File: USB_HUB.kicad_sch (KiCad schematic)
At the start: 2 parts, among them U1 TUSB8043A, Y1 Crystal_GND24

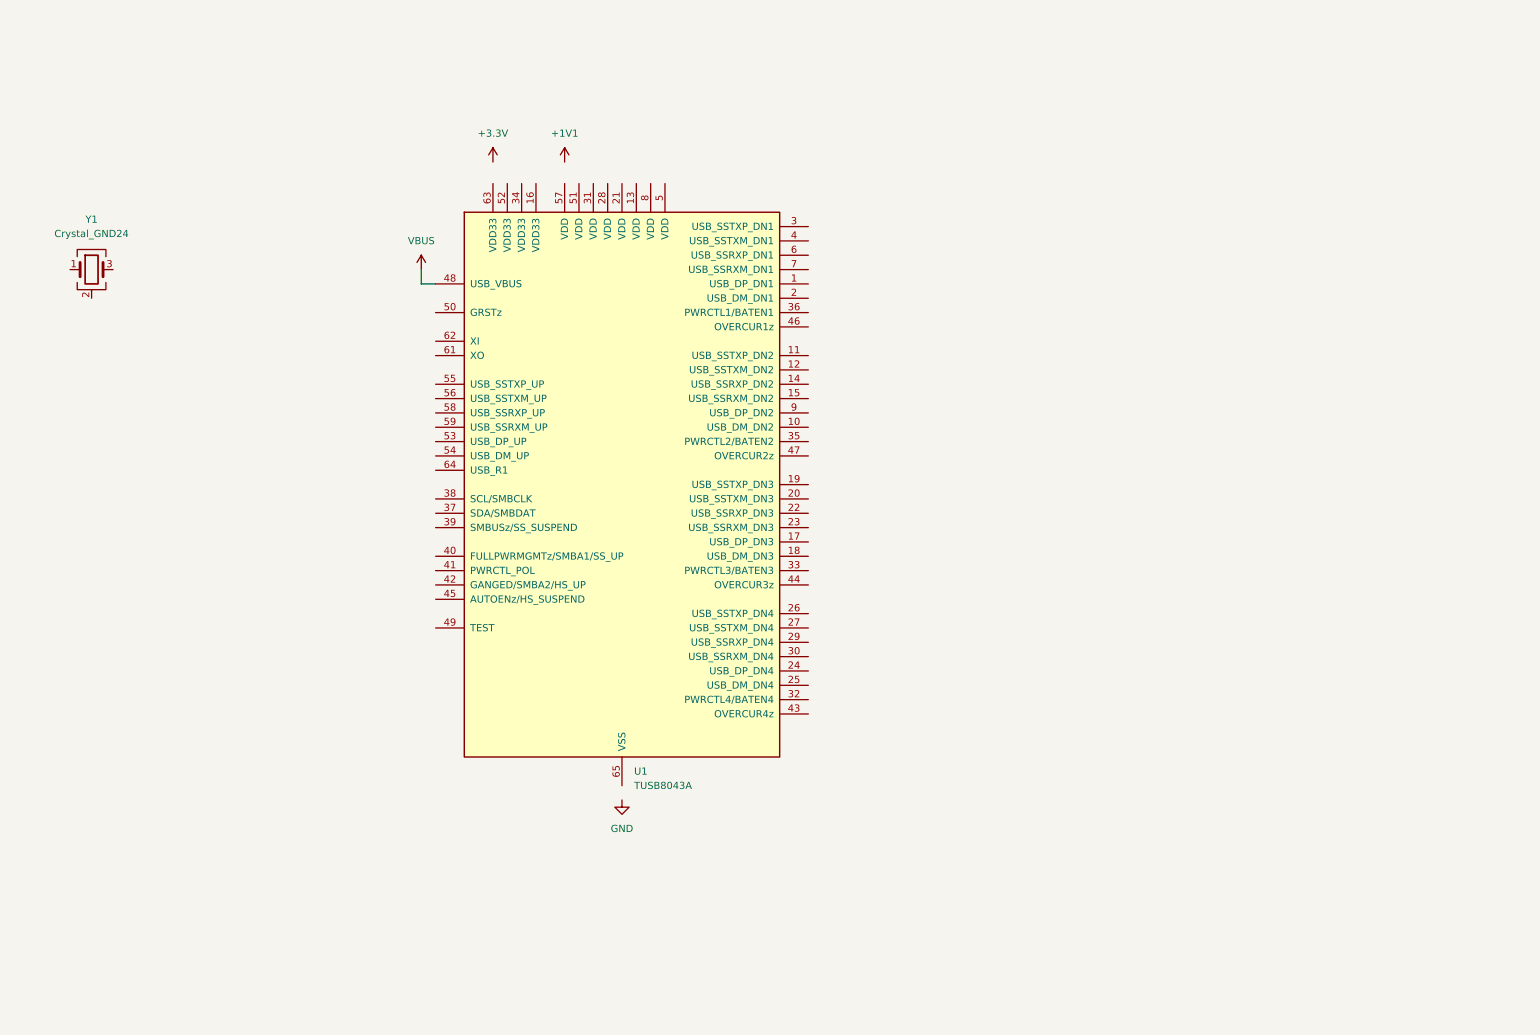
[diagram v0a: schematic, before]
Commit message: Weiter gearbeitet
Fast fertig:
HUB
Fertig
Connector (Up and Down)
MUX
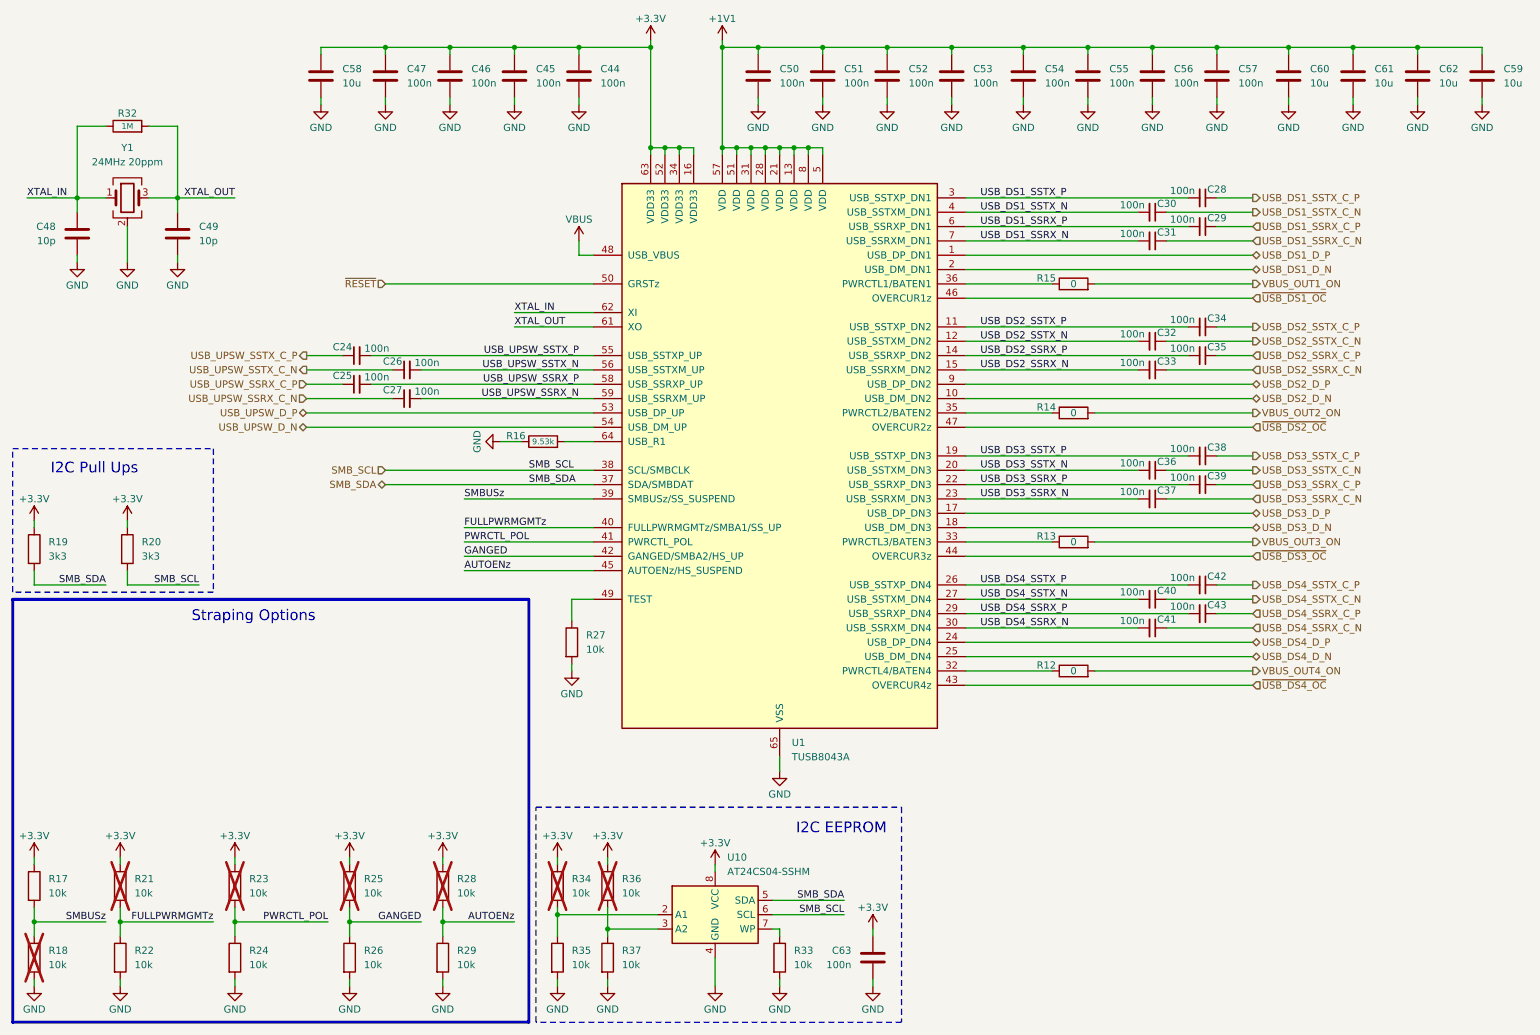
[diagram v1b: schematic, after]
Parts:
- added C24, C25, C26, C27, C28, C29, C30, C31, C32, C33, C34, C35, C36, C37, C38, C39, C40, C41, C42, C43: 100n, symbol Device:C_Small
- added C44, C45, C46, C47, C50, C51, C52, C53, C54, C55, C56, C57, C63: 100n, Capacitor_SMD:C_0402_1005Metric, symbol Device:C
- added C48, C49: 10p, Capacitor_SMD:C_0402_1005Metric, symbol Device:C
- added C58, C59, C60, C61, C62: 10u, Capacitor_SMD:C_0603_1608Metric, symbol Device:C
- added R12, R13, R14, R15: 0, Resistor_SMD:R_0402_1005Metric, symbol Device:R
- added R16: 9.53k, Resistor_SMD:R_0402_1005Metric, symbol Device:R
- added R17, R18, R21, R22, R23, R24, R25, R26, R27, R28, R29, R33, R34, R35, R36, R37: 10k, Resistor_SMD:R_0402_1005Metric, symbol Device:R
- added R19, R20: 3k3, Resistor_SMD:R_0402_1005Metric, symbol Device:R
- added R32: 1M, Resistor_SMD:R_0402_1005Metric, symbol Device:R
- added U10: AT24CS04-SSHM, Package_SO:SOIC-8_3.9x4.9mm_P1.27mm, symbol Memory_EEPROM:AT24CS04-SSHM
- Y1: value Crystal_GND24 -> 24MHz 20ppm
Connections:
- net +1V1: now also U1.13 (VDD), U1.21 (VDD), U1.28 (VDD), U1.31 (VDD), U1.5 (VDD), U1.51 (VDD), U1.57 (VDD), U1.8 (VDD), C50.2, C51.2, C52.2, C53.2, C54.2, C55.2, C56.2, C57.2, C59.1, C60.1, C61.1, C62.1
- net +3.3V: now also U1.16 (VDD33), U1.34 (VDD33), U1.52 (VDD33), U1.63 (VDD33), C44.2, C45.2, C46.2, C47.2, C58.1, C63.2, R17.1, R19.1, R20.1, R21.1, R23.1, R25.1, R28.1, R34.1, R36.1, U10.8 (VCC)
- net GND: now also U1.65 (VSS), Y1.2 (G), Y1.4 (G), C44.1, C45.1, C46.1, C47.1, C48.1, C49.1, C50.1, C51.1, C52.1, C53.1, C54.1, C55.1, C56.1, C57.1, C58.2, C59.2, C60.2, C61.2, C62.2, C63.1, R16.1, R18.2, R22.2, R24.2, R26.2, R27.2, R29.2, R33.2, R35.2, R37.2, U10.4 (GND)
- net USB_DS1_D_P: now reaches U1.1 (USB_DP_DN1)
- net USB_DS2_D_N: now reaches U1.10 (USB_DM_DN2)
- net USB_DS2_SSTX_P: now reaches U1.11 (USB_SSTXP_DN2)
- net USB_DS2_SSTX_P: now also C34.2
- net USB_DS2_SSTX_N: now reaches U1.12 (USB_SSTXM_DN2)
- net USB_DS2_SSTX_N: now also C32.2
- net USB_DS2_SSRX_P: now reaches U1.14 (USB_SSRXP_DN2)
- net USB_DS2_SSRX_P: now also C35.2
- net USB_DS2_SSRX_N: now reaches U1.15 (USB_SSRXM_DN2)
- net USB_DS2_SSRX_N: now also C33.2
- net USB_DS3_D_P: now reaches U1.17 (USB_DP_DN3)
- net USB_DS3_D_N: now reaches U1.18 (USB_DM_DN3)
- net USB_DS3_SSTX_P: now reaches U1.19 (USB_SSTXP_DN3)
- net USB_DS3_SSTX_P: now also C38.2
- net USB_DS1_D_N: now reaches U1.2 (USB_DM_DN1)
- net USB_DS3_SSTX_N: now reaches U1.20 (USB_SSTXM_DN3)
- net USB_DS3_SSTX_N: now also C36.2
- net USB_DS3_SSRX_P: now reaches U1.22 (USB_SSRXP_DN3)
- net USB_DS3_SSRX_P: now also C39.2
- net USB_DS3_SSRX_N: now reaches U1.23 (USB_SSRXM_DN3)
- net USB_DS3_SSRX_N: now also C37.2
- net USB_DS4_D_P: now reaches U1.24 (USB_DP_DN4)
- net USB_DS4_D_N: now reaches U1.25 (USB_DM_DN4)
- net USB_DS4_SSTX_P: now reaches U1.26 (USB_SSTXP_DN4)
- net USB_DS4_SSTX_P: now also C42.2
- net USB_DS4_SSTX_N: now reaches U1.27 (USB_SSTXM_DN4)
- net USB_DS4_SSTX_N: now also C40.2
- net USB_DS4_SSRX_P: now reaches U1.29 (USB_SSRXP_DN4)
- net USB_DS4_SSRX_P: now also C43.2
- net USB_DS1_SSTX_P: now reaches U1.3 (USB_SSTXP_DN1)
- net USB_DS1_SSTX_P: now also C28.2
- net USB_DS4_SSRX_N: now reaches U1.30 (USB_SSRXM_DN4)
- net USB_DS4_SSRX_N: now also C41.2
- net at U1.32 (PWRCTL4/BATEN4): now also R12.1
- net at U1.33 (PWRCTL3/BATEN3): now also R13.1
- net at U1.35 (PWRCTL2/BATEN2): now also R14.1
- net at U1.36 (PWRCTL1/BATEN1): now also R15.1
- net SMB_SDA: now reaches U1.37 (SDA/SMBDAT)
- net SMB_SDA: now also R19.2, U10.5 (SDA)
- net SMB_SCL: now reaches U1.38 (SCL/SMBCLK)
- net SMB_SCL: now also R20.2, U10.6 (SCL)
- net SMBUSz: now reaches U1.39 (SMBUSz/SS_SUSPEND)
- net SMBUSz: now also R17.2, R18.1
- net USB_DS1_SSTX_N: now reaches U1.4 (USB_SSTXM_DN1)
- net USB_DS1_SSTX_N: now also C30.2
- net FULLPWRMGMTz: now reaches U1.40 (FULLPWRMGMTz/SMBA1/SS_UP)
- net FULLPWRMGMTz: now also R21.2, R22.1
- net PWRCTL_POL: now reaches U1.41 (PWRCTL_POL)
- net PWRCTL_POL: now also R23.2, R24.1
- net GANGED: now reaches U1.42 (GANGED/SMBA2/HS_UP)
- net GANGED: now also R25.2, R26.1
- net ~{USB_DS4_OC}: now reaches U1.43 (OVERCUR4z)
- net ~{USB_DS3_OC}: now reaches U1.44 (OVERCUR3z)
- net AUTOENz: now reaches U1.45 (AUTOENz/HS_SUSPEND)
- net AUTOENz: now also R28.2, R29.1
- net ~{USB_DS1_OC}: now reaches U1.46 (OVERCUR1z)
- net ~{USB_DS2_OC}: now reaches U1.47 (OVERCUR2z)
- net at U1.49 (TEST): now also R27.1
- net ~{RESET}: now reaches U1.50 (GRSTz)
- net USB_UPSW_D_P: now reaches U1.53 (USB_DP_UP)
- net USB_UPSW_D_N: now reaches U1.54 (USB_DM_UP)
- net USB_UPSW_SSTX_P: now reaches U1.55 (USB_SSTXP_UP)
- net USB_UPSW_SSTX_P: now also C24.2
- net USB_UPSW_SSTX_N: now reaches U1.56 (USB_SSTXM_UP)
- net USB_UPSW_SSTX_N: now also C26.2
- net USB_UPSW_SSRX_P: now reaches U1.58 (USB_SSRXP_UP)
- net USB_UPSW_SSRX_P: now also C25.2
- net USB_UPSW_SSRX_N: now reaches U1.59 (USB_SSRXM_UP)
- net USB_UPSW_SSRX_N: now also C27.2
- net USB_DS1_SSRX_P: now reaches U1.6 (USB_SSRXP_DN1)
- net USB_DS1_SSRX_P: now also C29.2
- net XTAL_OUT: now reaches U1.61 (XO)
- net XTAL_OUT: now also Y1.3, C49.2, R32.2
- net XTAL_IN: now reaches U1.62 (XI)
- net XTAL_IN: now also Y1.1, C48.2, R32.1
- net at U1.64 (USB_R1): now also R16.2
- net USB_DS1_SSRX_N: now reaches U1.7 (USB_SSRXM_DN1)
- net USB_DS1_SSRX_N: now also C31.2
- net USB_DS2_D_P: now reaches U1.9 (USB_DP_DN2)
- new net: R34.2, R35.1, U10.2 (A1)
- new net: R36.2, R37.1, U10.3 (A2)
- new net: R33.1, U10.7 (WP)
- new net USB_DS1_SSRX_C_N: C31.1
- new net USB_DS1_SSRX_C_P: C29.1
- new net USB_DS1_SSTX_C_N: C30.1
- new net USB_DS1_SSTX_C_P: C28.1
- new net USB_DS2_SSRX_C_N: C33.1
- new net USB_DS2_SSRX_C_P: C35.1
- new net USB_DS2_SSTX_C_N: C32.1
- new net USB_DS2_SSTX_C_P: C34.1
- new net USB_DS3_SSRX_C_N: C37.1
- new net USB_DS3_SSRX_C_P: C39.1
- new net USB_DS3_SSTX_C_N: C36.1
- new net USB_DS3_SSTX_C_P: C38.1
- new net USB_DS4_SSRX_C_N: C41.1
- new net USB_DS4_SSRX_C_P: C43.1
- new net USB_DS4_SSTX_C_N: C40.1
- new net USB_DS4_SSTX_C_P: C42.1
- new net USB_UPSW_SSRX_C_N: C27.1
- new net USB_UPSW_SSRX_C_P: C25.1
- new net USB_UPSW_SSTX_C_N: C26.1
- new net USB_UPSW_SSTX_C_P: C24.1
- new net VBUS_OUT1_ON: R15.2
- new net VBUS_OUT2_ON: R14.2
- new net VBUS_OUT3_ON: R13.2
- new net VBUS_OUT4_ON: R12.2
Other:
- note added: "I2C EEPROM"
- note added: "I2C Pull Ups"
- note added: "Straping Options"
- moved on the sheet: U1, Y1

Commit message: Footprints Updated
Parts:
- C24, C25, C26, C27, C28, C29, C30, C31, C32, C33, C34, C35, C36, C37, C38, C39, C40, C41, C42, C43: footprint (none) -> 00_Capacitor:Cap_0402
- C44, C45, C46, C47, C48, C49, C50, C51, C52, C53, C54, C55, C56, C57, C63: footprint Capacitor_SMD:C_0402_1005Metric -> 00_Capacitor:Cap_0402
- C58, C59, C60, C61, C62: footprint Capacitor_SMD:C_0603_1608Metric -> 00_Capacitor:Cap_0603
- R12, R13, R14, R15, R16, R17, R18, R19, R20, R21, R22, R23, R24, R25, R26, R27, R28, R29, R32, R33, R34, R35, R36, R37: footprint Resistor_SMD:R_0402_1005Metric -> 00_Resistor:Res_0402
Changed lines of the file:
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@@
 			)
 		)
-		(property "Footprint" "Resistor_SMD:R_0402_1005Metric"
+		(property "Footprint" "00_Resistor:Res_0402"
 			(at 203.2 66.548 90)
 			(effects
@@
 			)
 		)
-		(property "Footprint" ""
+		(property "Footprint" "00_Capacitor:Cap_0402"
 			(at 217.17 57.15 0)
 			(effects
@@
 			)
 		)
-		(property "Footprint" ""
+		(property "Footprint" "00_Capacitor:Cap_0402"
 			(at 217.17 74.93 0)
 			(effects
@@
 			)
 		)
-		(property "Footprint" "Capacitor_SMD:C_0402_1005Metric"
+		(property "Footprint" "00_Capacitor:Cap_0402"
 			(at 43.4848 52.07 0)
 			(effects
@@
 			)
 		)
-		(property "Footprint" ""
+		(property "Footprint" "00_Capacitor:Cap_0402"
 			(at 217.17 80.01 0)
 			(effects
@@
 			)
 		)
-		(property "Footprint" "Capacitor_SMD:C_0402_1005Metric"
+		(property "Footprint" "00_Capacitor:Cap_0402"
 			(at 80.3148 24.13 0)
 			(effects
@@
 			)
 		)
-		(property "Footprint" "Resistor_SMD:R_0402_1005Metric"
+		(property "Footprint" "00_Resistor:Res_0402"
 			(at 73.152 171.45 90)
 			(effects
@@
 			)
 		)
-		(property "Footprint" "Resistor_SMD:R_0402_1005Metric"
+		(property "Footprint" "00_Resistor:Res_0402"
 			(at 52.832 184.15 90)
 			(effects
@@
 			)
 		)
-		(property "Footprint" ""
+		(property "Footprint" "00_Capacitor:Cap_0402"
 			(at 85.09 85.09 0)
 			(effects
@@
 			)
 		)
-		(property "Footprint" "Resistor_SMD:R_0402_1005Metric"
+		(property "Footprint" "00_Resistor:Res_0402"
 			(at 17.272 111.76 90)
 			(effects
@@
 			)
 		)
-		(property "Footprint" "Capacitor_SMD:C_0402_1005Metric"
+		(property "Footprint" "00_Capacitor:Cap_0402"
 			(at 157.7848 24.13 0)
 			(effects
@@
 			)
 		)
-		(property "Footprint" "Resistor_SMD:R_0402_1005Metric"
+		(property "Footprint" "00_Resistor:Res_0402"
 			(at 32.512 171.45 90)
 			(effects
@@
 			)
 		)
-		(property "Footprint" "Resistor_SMD:R_0402_1005Metric"
+		(property "Footprint" "00_Resistor:Res_0402"
 			(at 109.982 171.45 90)
 			(effects
@@
 			)
 		)
-		(property "Footprint" "Resistor_SMD:R_0402_1005Metric"
+		(property "Footprint" "00_Resistor:Res_0402"
 			(at 17.272 184.15 90)
 			(effects
@@
 			)
 		)
-		(property "Footprint" "Resistor_SMD:R_0402_1005Metric"
+		(property "Footprint" "00_Resistor:Res_0402"
 			(at 149.352 184.15 90)
 			(effects
@@
 			)
 		)
-		(property "Footprint" ""
+		(property "Footprint" "00_Capacitor:Cap_0402"
 			(at 217.17 102.87 0)
 			(effects
@@
 			)
 		)
-		(property "Footprint" "Capacitor_SMD:C_0603_1608Metric"
+		(property "Footprint" "00_Capacitor:Cap_0603"
 			(at 253.6952 31.75 0)
 			(effects
@@
 			)
 		)
-		(property "Footprint" ""
+		(property "Footprint" "00_Capacitor:Cap_0402"
 			(at 217.17 120.65 0)
 			(effects
@@
 			)
 		)
-		(property "Footprint" ""
+		(property "Footprint" "00_Capacitor:Cap_0402"
 			(at 226.06 77.47 0)
 			(effects
@@
 			)
 		)
-		(property "Footprint" "Capacitor_SMD:C_0402_1005Metric"
+		(property "Footprint" "00_Capacitor:Cap_0402"
 			(at 103.1748 24.13 0)
 			(effects
@@
 			)
 		)
-		(property "Footprint" "Capacitor_SMD:C_0402_1005Metric"
+		(property "Footprint" "00_Capacitor:Cap_0402"
 			(at 168.6052 180.34 0)
 			(effects
@@
 			)
 		)
-		(property "Footprint" "Capacitor_SMD:C_0603_1608Metric"
+		(property "Footprint" "00_Capacitor:Cap_0603"
 			(at 265.1252 31.75 0)
 			(effects
@@
 			)
 		)
-		(property "Footprint" ""
+		(property "Footprint" "00_Capacitor:Cap_0402"
 			(at 76.2 82.55 0)
 			(effects
@@
 			)
 		)
-		(property "Footprint" "Capacitor_SMD:C_0603_1608Metric"
+		(property "Footprint" "00_Capacitor:Cap_0603"
 			(at 242.2652 31.75 0)
 			(effects
@@
 			)
 		)
-		(property "Footprint" "Capacitor_SMD:C_0402_1005Metric"
+		(property "Footprint" "00_Capacitor:Cap_0402"
 			(at 114.6048 24.13 0)
 			(effects
@@
 			)
 		)
-		(property "Footprint" "Resistor_SMD:R_0402_1005Metric"
+		(property "Footprint" "00_Resistor:Res_0402"
 			(at 32.512 184.15 90)
 			(effects
@@
 			)
 		)
-		(property "Footprint" "Capacitor_SMD:C_0402_1005Metric"
+		(property "Footprint" "00_Capacitor:Cap_0402"
 			(at 216.2048 24.13 0)
 			(effects
@@
 			)
 		)
-		(property "Footprint" "Capacitor_SMD:C_0402_1005Metric"
+		(property "Footprint" "00_Capacitor:Cap_0402"
 			(at 204.7748 24.13 0)
 			(effects
@@
 			)
 		)
-		(property "Footprint" "Capacitor_SMD:C_0402_1005Metric"
+		(property "Footprint" "00_Capacitor:Cap_0402"
 			(at 180.6448 24.13 0)
 			(effects
@@
 			)
 		)
-		(property "Footprint" "Resistor_SMD:R_0402_1005Metric"
+		(property "Footprint" "00_Resistor:Res_0402"
 			(at 109.982 184.15 90)
 			(effects
@@
 			)
 		)
-		(property "Footprint" "Capacitor_SMD:C_0603_1608Metric"
+		(property "Footprint" "00_Capacitor:Cap_0603"
 			(at 70.8152 31.75 0)
 			(effects
@@
 			)
 		)
-		(property "Footprint" "Resistor_SMD:R_0402_1005Metric"
+		(property "Footprint" "00_Resistor:Res_0402"
 			(at 35.56 38.608 90)
 			(effects
@@
 			)
 		)
-		(property "Footprint" "Resistor_SMD:R_0402_1005Metric"
+		(property "Footprint" "00_Resistor:Res_0402"
 			(at 17.272 171.45 90)
 			(effects
@@
 			)
 		)
-		(property "Footprint" ""
+		(property "Footprint" "00_Capacitor:Cap_0402"
 			(at 217.17 52.07 0)
 			(effects
@@
 			)
 		)
-		(property "Footprint" "Capacitor_SMD:C_0402_1005Metric"
+		(property "Footprint" "00_Capacitor:Cap_0402"
 			(at 169.2148 24.13 0)
 			(effects
@@
 			)
 		)
-		(property "Footprint" ""
+		(property "Footprint" "00_Capacitor:Cap_0402"
 			(at 217.17 125.73 0)
 			(effects
@@
 			)
 		)
-		(property "Footprint" "Capacitor_SMD:C_0402_1005Metric"
+		(property "Footprint" "00_Capacitor:Cap_0402"
 			(at 193.3448 24.13 0)
 			(effects
@@
 			)
 		)
-		(property "Footprint" "Capacitor_SMD:C_0402_1005Metric"
+		(property "Footprint" "00_Capacitor:Cap_0402"
 			(at 227.6348 24.13 0)
 			(effects
@@
 			)
 		)
-		(property "Footprint" ""
+		(property "Footprint" "00_Capacitor:Cap_0402"
 			(at 226.06 118.11 0)
 			(effects
@@
 			)
 		)
-		(property "Footprint" "Resistor_SMD:R_0402_1005Metric"
+		(property "Footprint" "00_Resistor:Res_0402"
 			(at 73.152 184.15 90)
 			(effects
@@
 			)
 		)
-		(property "Footprint" "Resistor_SMD:R_0402_1005Metric"
+		(property "Footprint" "00_Resistor:Res_0402"
 			(at 109.22 94.488 90)
 			(effects
@@
 			)
 		)
-		(property "Footprint" "Resistor_SMD:R_0402_1005Metric"
+		(property "Footprint" "00_Resistor:Res_0402"
 			(at 203.2 89.408 90)
 			(effects
@@
 			)
 		)
-		(property "Footprint" "Resistor_SMD:R_0402_1005Metric"
+		(property "Footprint" "00_Resistor:Res_0402"
 			(at 52.832 171.45 90)
 			(effects
@@
 			)
 		)
-		(property "Footprint" "Capacitor_SMD:C_0402_1005Metric"
+		(property "Footprint" "00_Capacitor:Cap_0402"
 			(at 146.3548 24.13 0)
 			(effects
@@
 			)
 		)
-		(property "Footprint" ""
+		(property "Footprint" "00_Capacitor:Cap_0402"
 			(at 226.06 72.39 0)
 			(effects
@@
 			)
 		)
-		(property "Footprint" "Capacitor_SMD:C_0402_1005Metric"
+		(property "Footprint" "00_Capacitor:Cap_0402"
 			(at 27.6352 52.07 0)
 			(effects
@@
 			)
 		)
-		(property "Footprint" ""
+		(property "Footprint" "00_Capacitor:Cap_0402"
 			(at 226.06 54.61 0)
 			(effects
@@
 			)
 		)
-		(property "Footprint" "Capacitor_SMD:C_0402_1005Metric"
+		(property "Footprint" "00_Capacitor:Cap_0402"
 			(at 91.7448 24.13 0)
 			(effects
@@
 			)
 		)
-		(property "Footprint" ""
+		(property "Footprint" "00_Capacitor:Cap_0402"
 			(at 217.17 97.79 0)
 			(effects
@@
 			)
 		)
-		(property "Footprint" ""
+		(property "Footprint" "00_Capacitor:Cap_0402"
 			(at 226.06 49.53 0)
 			(effects
@@
 			)
 		)
-		(property "Footprint" "Resistor_SMD:R_0402_1005Metric"
+		(property "Footprint" "00_Resistor:Res_0402"
 			(at 89.662 171.45 90)
 			(effects
@@
 			)
 		)
-		(property "Footprint" ""
+		(property "Footprint" "00_Capacitor:Cap_0402"
 			(at 226.06 95.25 0)
 			(effects
@@
 			)
 		)
-		(property "Footprint" ""
+		(property "Footprint" "00_Capacitor:Cap_0402"
 			(at 226.06 123.19 0)
 			(effects
@@
 			)
 		)
-		(property "Footprint" "Resistor_SMD:R_0402_1005Metric"
+		(property "Footprint" "00_Resistor:Res_0402"
 			(at 203.2 112.268 90)
 			(effects
@@
 			)
 		)
-		(property "Footprint" "Resistor_SMD:R_0402_1005Metric"
+		(property "Footprint" "00_Resistor:Res_0402"
 			(at 33.782 111.76 90)
 			(effects
@@
 			)
 		)
-		(property "Footprint" "Resistor_SMD:R_0402_1005Metric"
+		(property "Footprint" "00_Resistor:Res_0402"
 			(at 118.872 184.15 90)
 			(effects
@@
 			)
 		)
-		(property "Footprint" "Resistor_SMD:R_0402_1005Metric"
+		(property "Footprint" "00_Resistor:Res_0402"
 			(at 89.662 184.15 90)
 			(effects
@@
 			)
 		)
-		(property "Footprint" "Resistor_SMD:R_0402_1005Metric"
+		(property "Footprint" "00_Resistor:Res_0402"
 			(at 112.522 128.27 90)
 			(effects
@@
 			)
 		)
-		(property "Footprint" ""
+		(property "Footprint" "00_Capacitor:Cap_0402"
 			(at 85.09 80.01 0)
 			(effects
@@
 			)
 		)
-		(property "Footprint" "Resistor_SMD:R_0402_1005Metric"
+		(property "Footprint" "00_Resistor:Res_0402"
 			(at 118.872 171.45 90)
 			(effects
@@
 			)
 		)
-		(property "Footprint" ""
+		(property "Footprint" "00_Capacitor:Cap_0402"
 			(at 76.2 77.47 0)
 			(effects
@@
 			)
 		)
-		(property "Footprint" ""
+		(property "Footprint" "00_Capacitor:Cap_0402"
 			(at 226.06 100.33 0)
 			(effects
@@
 			)
 		)
-		(property "Footprint" "Capacitor_SMD:C_0603_1608Metric"
+		(property "Footprint" "00_Capacitor:Cap_0603"
 			(at 276.5552 31.75 0)
 			(effects
@@
 			)
 		)
-		(property "Footprint" "Resistor_SMD:R_0402_1005Metric"
+		(property "Footprint" "00_Resistor:Res_0402"
 			(at 203.2 135.128 90)
 			(effects
